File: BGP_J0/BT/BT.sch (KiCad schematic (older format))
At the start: 20 parts, among them P1 CONN_01X02, P2 CONN_01X02, P3 CONN_01X04, P4 CONN_01X04, Q1 MMBF5457

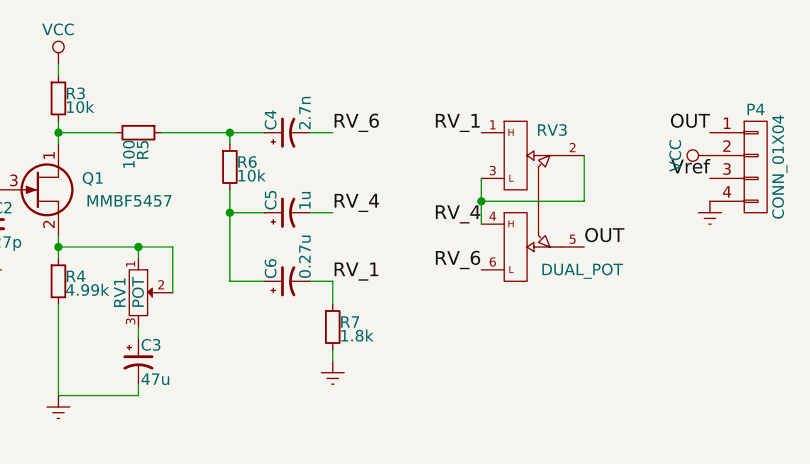
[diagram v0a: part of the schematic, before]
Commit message: Some Changes
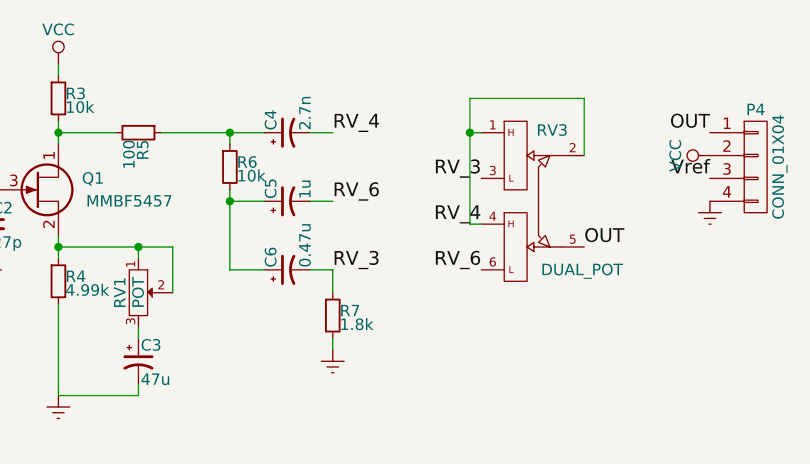
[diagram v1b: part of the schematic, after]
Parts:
- C6: value 0.27u -> 0.47u
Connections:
- net RV_4: now also C4.2, RV3.1; no longer C5.2, RV3.3
- net RV_6: now also C5.2; no longer C4.2
- net RV_1 renamed RV_3
- net RV_3: now also RV3.3; no longer RV3.1
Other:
- moved on the sheet: C5, C6, R7
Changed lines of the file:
@@
 $EndComp
 $Comp
-L Earth #PWR4
+L Earth #PWR01
 U 1 1 5A6FCA5D
 P 4300 3900
-F 0 "#PWR4" H 4300 3650 50  0001 C CNN
+F 0 "#PWR01" H 4300 3650 50  0001 C CNN
 F 1 "Earth" H 4300 3750 50  0001 C CNN
 F 2 "" H 4300 3900 50  0000 C CNN
@@
 $EndComp
 $Comp
-L Earth #PWR5
+L Earth #PWR02
 U 1 1 5A6FCA7B
 P 5100 3900
-F 0 "#PWR5" H 5100 3650 50  0001 C CNN
+F 0 "#PWR02" H 5100 3650 50  0001 C CNN
 F 1 "Earth" H 5100 3750 50  0001 C CNN
 F 2 "" H 5100 3900 50  0000 C CNN
@@
 	5400 3100 5400 3050
 $Comp
-L VCC #PWR6
+L VCC #PWR03
 U 1 1 5A6FCE1E
 P 5400 3050
-F 0 "#PWR6" H 5400 2900 50  0001 C CNN
+F 0 "#PWR03" H 5400 2900 50  0001 C CNN
 F 1 "VCC" H 5400 3200 50  0000 C CNN
 F 2 "" H 5400 3050 50  0000 C CNN
@@
 L CP1_Small C5
 U 1 1 5A6FD2DA
-P 6400 3700
-F 0 "C5" H 6410 3770 50  0000 L CNN
-F 1 "1u" H 6410 3620 50  0000 L CNN
-F 2 "Capacitors_Tantalum_SMD:TantalC_SizeR_EIA-2012" H 6400 3700 50  0001 C CNN
-F 3 "" H 6400 3700 50  0000 C CNN
-	1    6400 3700
+P 6400 3650
+F 0 "C5" H 6410 3720 50  0000 L CNN
+F 1 "1u" H 6410 3570 50  0000 L CNN
+F 2 "Capacitors_Tantalum_SMD:TantalC_SizeR_EIA-2012" H 6400 3650 50  0001 C CNN
+F 3 "" H 6400 3650 50  0000 C CNN
+	1    6400 3650
 	0    -1   -1   0
 $EndComp
@@
 L CP1_Small C6
 U 1 1 5A6FD31E
-P 6400 4000
-F 0 "C6" H 6410 4070 50  0000 L CNN
-F 1 "0.27u" H 6410 3920 50  0000 L CNN
-F 2 "Capacitors_Tantalum_SMD:TantalC_SizeR_EIA-2012" H 6400 4000 50  0001 C CNN
-F 3 "" H 6400 4000 50  0000 C CNN
-	1    6400 4000
+P 6400 3950
+F 0 "C6" H 6410 4020 50  0000 L CNN
+F 1 "0.47u" H 6410 3870 50  0000 L CNN
+F 2 "Capacitors_Tantalum_SMD:TantalC_SizeR_EIA-2012" H 6400 3950 50  0001 C CNN
+F 3 "" H 6400 3950 50  0000 C CNN
+	1    6400 3950
 	0    -1   -1   0
 $EndComp
 $Comp
-L Earth #PWR8
+L Earth #PWR04
 U 1 1 5A6FD3C7
-P 6600 4350
-F 0 "#PWR8" H 6600 4100 50  0001 C CNN
-F 1 "Earth" H 6600 4200 50  0001 C CNN
-F 2 "" H 6600 4350 50  0000 C CNN
-F 3 "" H 6600 4350 50  0000 C CNN
-	1    6600 4350
+P 6600 4300
+F 0 "#PWR04" H 6600 4050 50  0001 C CNN
+F 1 "Earth" H 6600 4150 50  0001 C CNN
+F 2 "" H 6600 4300 50  0000 C CNN
+F 3 "" H 6600 4300 50  0000 C CNN
+	1    6600 4300
 	1    0    0    -1
 $EndComp
@@
 Connection ~ 6150 3350
 Wire Wire Line
-	6150 3600 6150 4000
-Wire Wire Line
-	6150 3700 6300 3700
-Wire Wire Line
-	6150 4000 6300 4000
-Connection ~ 6150 3700
-Wire Wire Line
-	6600 4100 6600 4000
-Wire Wire Line
-	6600 3700 6500 3700
+	6150 3650 6300 3650
+Wire Wire Line
+	6150 3950 6300 3950
+Connection ~ 6150 3650
+Wire Wire Line
+	6600 4050 6600 3950
+Wire Wire Line
+	6600 3650 6500 3650
 Wire Wire Line
 	6600 3350 6500 3350
-Text Label 6600 3700 0    60   ~ 0
+Text Label 6600 3350 0    60   ~ 0
 RV_4
-Text Label 6600 3350 0    60   ~ 0
+Text Label 6600 3650 0    60   ~ 0
 RV_6
 Text Label 7700 3850 0    60   ~ 0
@@
 Text Label 7250 3950 2    60   ~ 0
 RV_6
-Wire Wire Line
-	7250 3550 7250 3750
-Wire Wire Line
-	7250 3650 7700 3650
-Wire Wire Line
-	7700 3650 7700 3450
-Text Label 6600 4000 0    60   ~ 0
-RV_1
-Connection ~ 7250 3650
-Text Label 7250 3350 2    60   ~ 0
-RV_1
-Wire Wire Line
-	6600 4350 6600 4300
+Text Label 6600 3950 0    60   ~ 0
+RV_3
+Wire Wire Line
+	6600 4300 6600 4250
 Text Label 4300 3600 2    60   ~ 0
 IN
@@
 Vref
 $Comp
-L Earth #PWR10
+L Earth #PWR05
 U 1 1 5A6FE42E
 P 8250 3650
-F 0 "#PWR10" H 8250 3400 50  0001 C CNN
+F 0 "#PWR05" H 8250 3400 50  0001 C CNN
 F 1 "Earth" H 8250 3500 50  0001 C CNN
 F 2 "" H 8250 3650 50  0000 C CNN
@@
 $EndComp
 $Comp
-L VCC #PWR9
+L VCC #PWR06
 U 1 1 5A6FE538
 P 8250 3450
-F 0 "#PWR9" H 8250 3300 50  0001 C CNN
+F 0 "#PWR06" H 8250 3300 50  0001 C CNN
 F 1 "VCC" H 8250 3600 50  0000 C CNN
 F 2 "" H 8250 3450 50  0000 C CNN
@@
 IN_N
 $Comp
-L Earth #PWR1
+L Earth #PWR07
 U 1 1 5A6FE8A6
 P 3650 3400
-F 0 "#PWR1" H 3650 3150 50  0001 C CNN
+F 0 "#PWR07" H 3650 3150 50  0001 C CNN
 F 1 "Earth" H 3650 3250 50  0001 C CNN
 F 2 "" H 3650 3400 50  0000 C CNN
@@
 $EndComp
 $Comp
-L Earth #PWR2
+L Earth #PWR08
 U 1 1 5A6FE8EA
 P 3650 3900
-F 0 "#PWR2" H 3650 3650 50  0001 C CNN
+F 0 "#PWR08" H 3650 3650 50  0001 C CNN
 F 1 "Earth" H 3650 3750 50  0001 C CNN
 F 2 "" H 3650 3900 50  0000 C CNN
@@
 IN
 $Comp
-L Earth #PWR7
+L Earth #PWR09
 U 1 1 5A6FF586
 P 5400 4500
-F 0 "#PWR7" H 5400 4250 50  0001 C CNN
+F 0 "#PWR09" H 5400 4250 50  0001 C CNN
 F 1 "Earth" H 5400 4350 50  0001 C CNN
 F 2 "" H 5400 4500 50  0000 C CNN
@@
 L R_Small R7
 U 1 1 5A6FDA7A
-P 6600 4200
-F 0 "R7" H 6630 4220 50  0000 L CNN
-F 1 "1.8k" H 6630 4160 50  0000 L CNN
-F 2 "Resistors_SMD:R_0603_HandSoldering" H 6600 4200 50  0001 C CNN
-F 3 "" H 6600 4200 50  0000 C CNN
-	1    6600 4200
-	1    0    0    -1
-$EndComp
-Wire Wire Line
-	6600 4000 6500 4000
-$Comp
-L Earth #PWR3
+P 6600 4150
+F 0 "R7" H 6630 4170 50  0000 L CNN
+F 1 "1.8k" H 6630 4110 50  0000 L CNN
+F 2 "Resistors_SMD:R_0603_HandSoldering" H 6600 4150 50  0001 C CNN
+F 3 "" H 6600 4150 50  0000 C CNN
+	1    6600 4150
+	1    0    0    -1
+$EndComp
+Wire Wire Line
+	6600 3950 6500 3950
+$Comp
+L Earth #PWR010
 U 1 1 5A713616
 P 3650 4600
-F 0 "#PWR3" H 3650 4350 50  0001 C CNN
+F 0 "#PWR010" H 3650 4350 50  0001 C CNN
 F 1 "Earth" H 3650 4450 50  0001 C CNN
 F 2 "" H 3650 4600 50  0000 C CNN
@@
 	1    0    0    -1
 $EndComp
+Text Label 7250 3550 2    60   ~ 0
+RV_3
+Wire Wire Line
+	7700 3450 7700 3200
+Wire Wire Line
+	7700 3200 7200 3200
+Wire Wire Line
+	7200 3200 7200 3750
+Wire Wire Line
+	7200 3350 7250 3350
+Wire Wire Line
+	7200 3750 7250 3750
+Connection ~ 7200 3350
+Wire Wire Line
+	6150 3600 6150 3950
 $EndSCHEMATC
